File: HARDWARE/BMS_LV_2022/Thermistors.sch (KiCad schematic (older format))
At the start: 18 parts

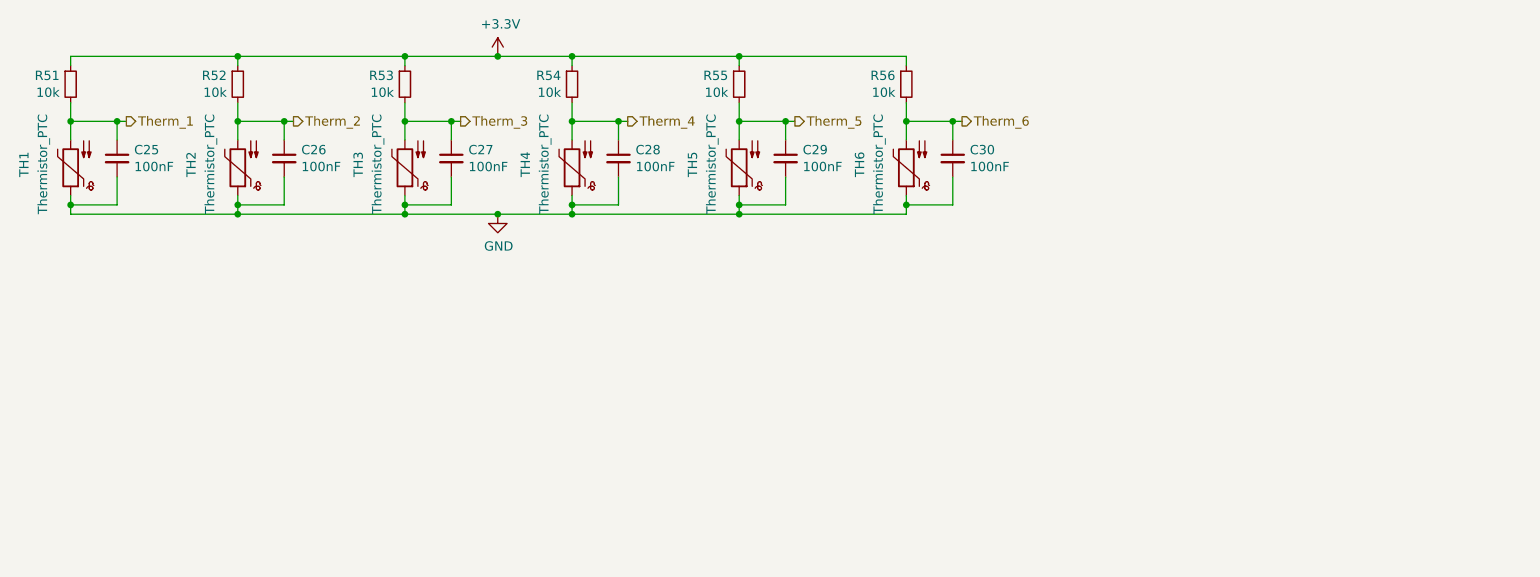
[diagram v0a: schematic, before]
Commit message: Most of the footprints added
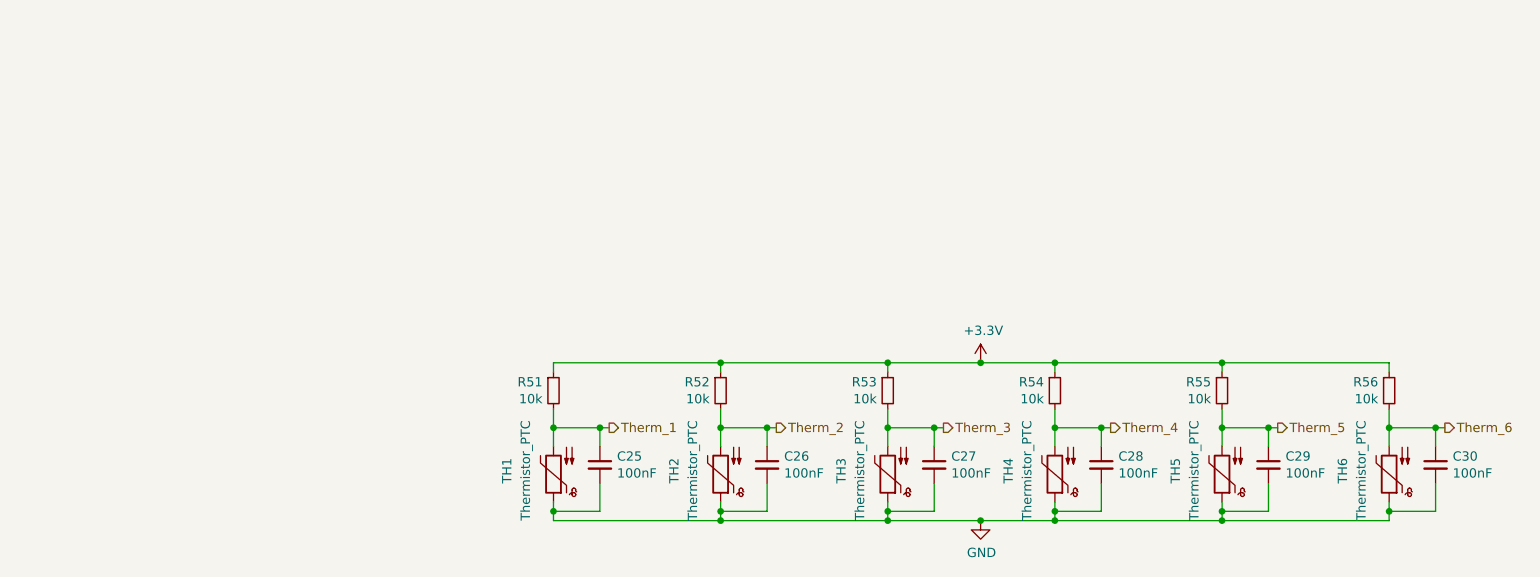
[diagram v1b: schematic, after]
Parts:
- C25, C26, C27, C28, C29, C30: footprint (none) -> Capacitor_SMD:C_0603_1608Metric
- R51, R52, R53, R54, R55, R56: footprint (none) -> Resistor_SMD:R_0603_1608Metric
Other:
- moved on the sheet: C25, C26, C27, C28, C29, C30, R51, R52, R53, R54, R55, R56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

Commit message: PCB layout init
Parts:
- TH1, TH2, TH3, TH4, TH5, TH6: footprint (none) -> Connector_PinHeader_2.54mm:PinHeader_1x02_P2.54mm_Vertical
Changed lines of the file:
@@
 F 0 "TH2" V 4800 4300 50  0000 R CNN
 F 1 "Thermistor_PTC" V 4700 4500 50  0000 R CNN
-F 2 "" H 4600 4050 50  0001 L CNN
+F 2 "Connector_PinHeader_2.54mm:PinHeader_1x02_P2.54mm_Vertical" H 4600 4050 50  0001 L CNN
 F 3 "~" H 4550 4250 50  0001 C CNN
 	1    4550 4250
@@
 F 0 "TH3" V 5700 4300 50  0000 R CNN
 F 1 "Thermistor_PTC" V 5600 4500 50  0000 R CNN
-F 2 "" H 5500 4050 50  0001 L CNN
+F 2 "Connector_PinHeader_2.54mm:PinHeader_1x02_P2.54mm_Vertical" H 5500 4050 50  0001 L CNN
 F 3 "~" H 5450 4250 50  0001 C CNN
 	1    5450 4250
@@
 F 0 "TH6" V 8400 4300 50  0000 R CNN
 F 1 "Thermistor_PTC" V 8300 4500 50  0000 R CNN
-F 2 "" H 8200 4050 50  0001 L CNN
+F 2 "Connector_PinHeader_2.54mm:PinHeader_1x02_P2.54mm_Vertical" H 8200 4050 50  0001 L CNN
 F 3 "~" H 8150 4250 50  0001 C CNN
 	1    8150 4250
@@
 F 0 "TH5" V 7500 4300 50  0000 R CNN
 F 1 "Thermistor_PTC" V 7400 4500 50  0000 R CNN
-F 2 "" H 7300 4050 50  0001 L CNN
+F 2 "Connector_PinHeader_2.54mm:PinHeader_1x02_P2.54mm_Vertical" H 7300 4050 50  0001 L CNN
 F 3 "~" H 7250 4250 50  0001 C CNN
 	1    7250 4250
@@
 F 0 "TH4" V 6600 4300 50  0000 R CNN
 F 1 "Thermistor_PTC" V 6500 4500 50  0000 R CNN
-F 2 "" H 6400 4050 50  0001 L CNN
+F 2 "Connector_PinHeader_2.54mm:PinHeader_1x02_P2.54mm_Vertical" H 6400 4050 50  0001 L CNN
 F 3 "~" H 6350 4250 50  0001 C CNN
 	1    6350 4250
@@
 F 0 "TH1" V 3900 4300 50  0000 R CNN
 F 1 "Thermistor_PTC" V 3800 4500 50  0000 R CNN
-F 2 "" H 3700 4050 50  0001 L CNN
+F 2 "Connector_PinHeader_2.54mm:PinHeader_1x02_P2.54mm_Vertical" H 3700 4050 50  0001 L CNN
 F 3 "~" H 3650 4250 50  0001 C CNN
 	1    3650 4250
